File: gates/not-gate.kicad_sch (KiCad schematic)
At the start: 5 parts, among them Q7 NPN, Q8 NPN

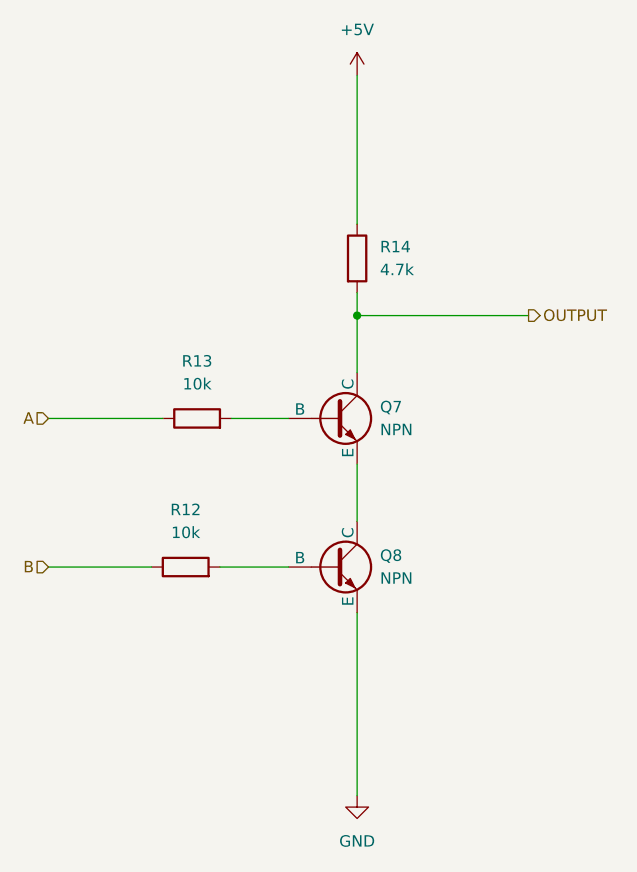
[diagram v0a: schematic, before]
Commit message: Schematic for register
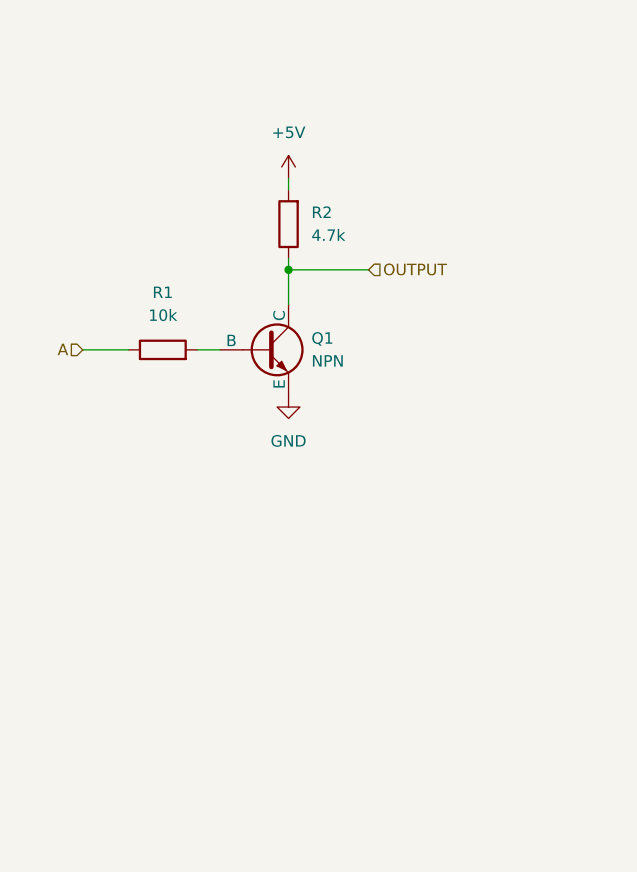
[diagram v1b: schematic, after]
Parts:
- removed Q7, Q8: NPN, symbol Simulation_SPICE:NPN
- removed R12, R13: 10k, Resistor_SMD:R_0201_0603Metric, symbol Device:R
- removed R14: 4.7k, Resistor_SMD:R_0201_0603Metric, symbol Device:R
- added Q1: NPN, symbol Simulation_SPICE:NPN
- added R1: 10k, symbol Device:R
- added R2: 4.7k, symbol Device:R
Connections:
- net +5V: now also R2.2
- net A: now also R1.1
- net GND: now also Q1.3 (E)
- net OUTPUT: now also Q1.1 (C), R2.1
- new net: Q1.2 (B), R1.2
